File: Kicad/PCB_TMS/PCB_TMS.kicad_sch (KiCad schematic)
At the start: 3 parts

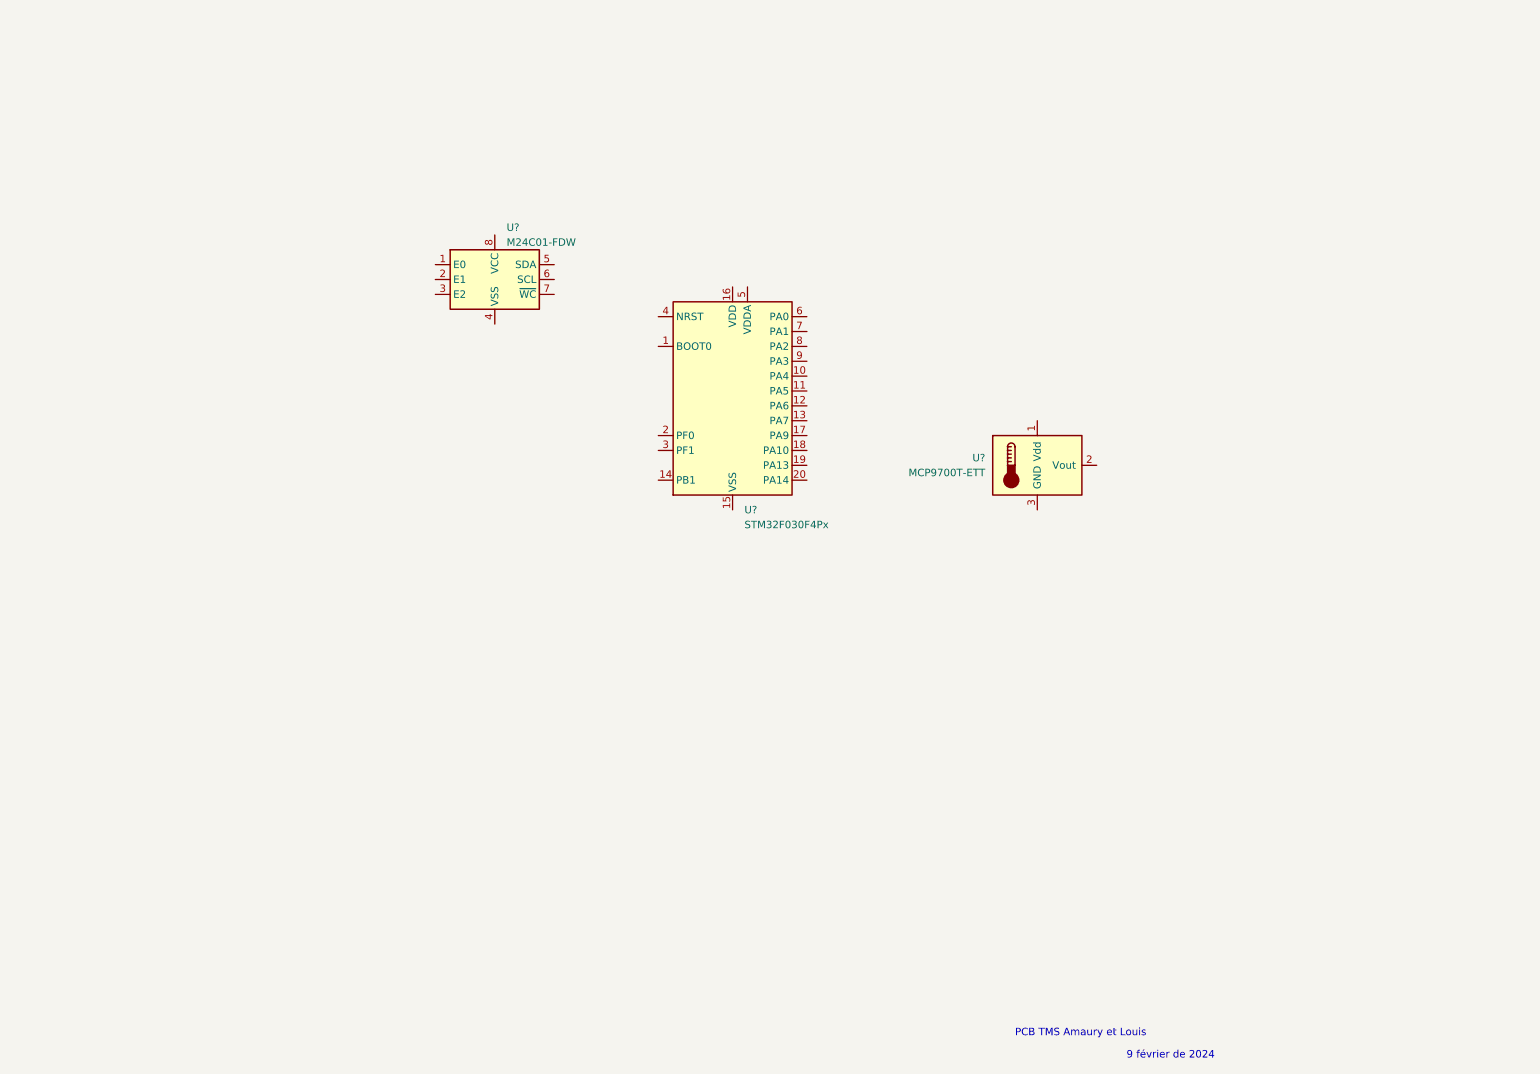
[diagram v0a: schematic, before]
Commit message: Fin schematic
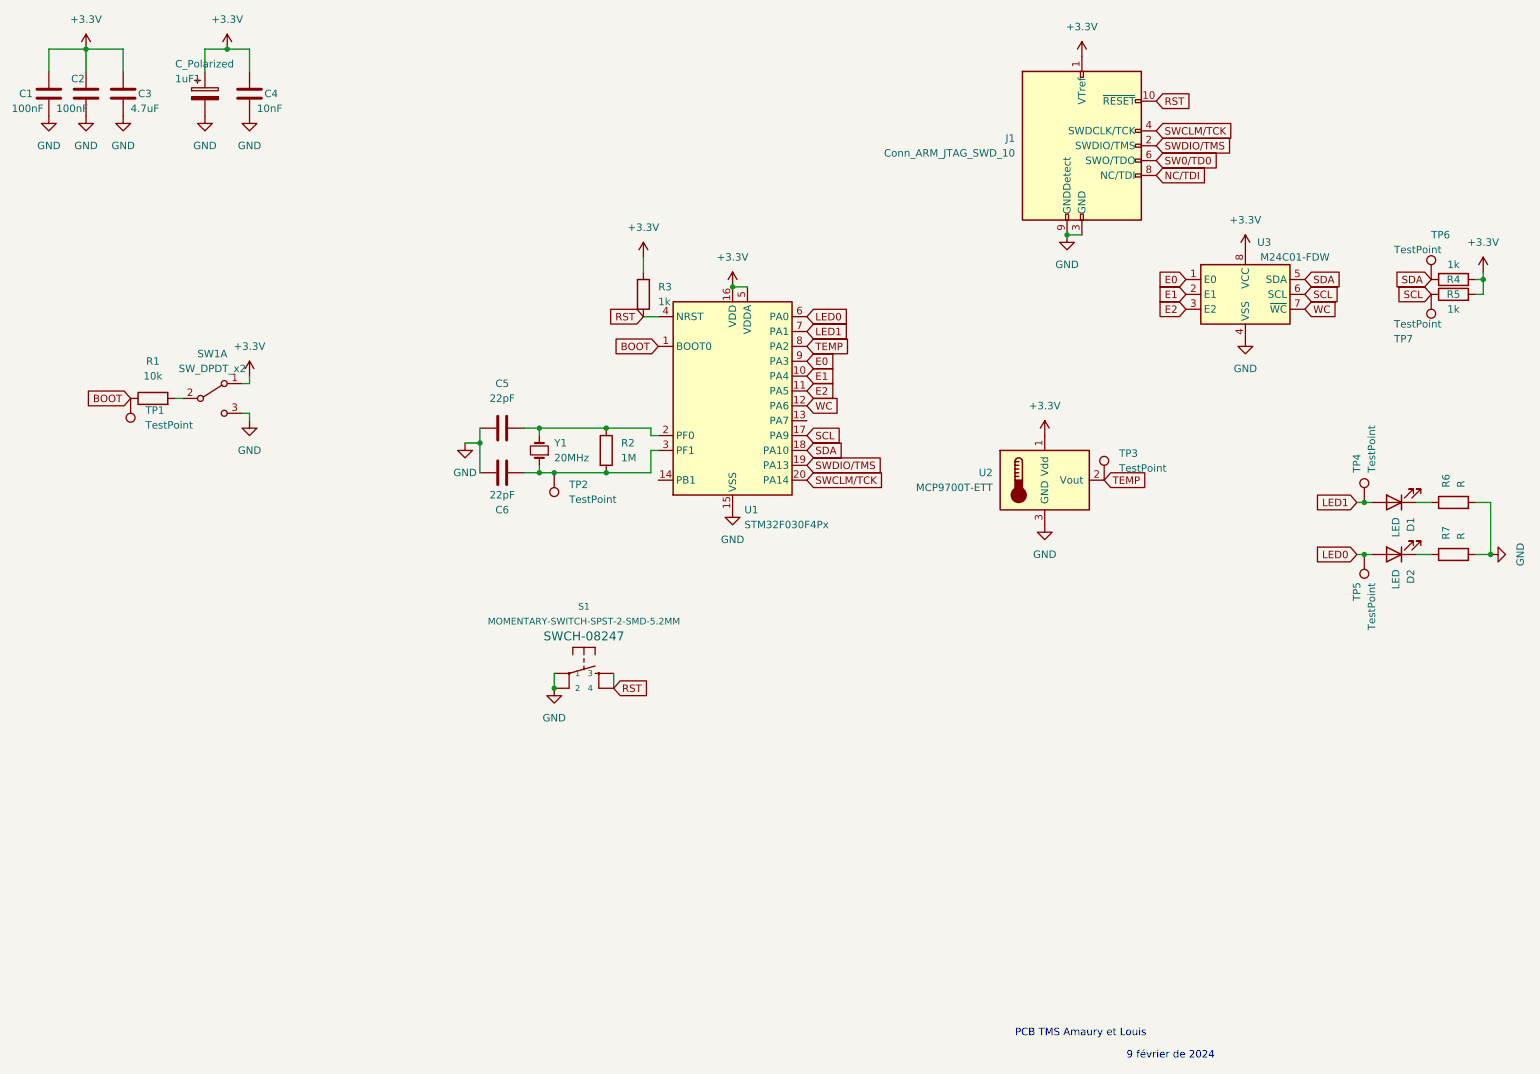
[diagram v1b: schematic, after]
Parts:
- added 1uF1: C_Polarized, symbol Device:C_Polarized
- added C1, C2: 100nF, Capacitor_SMD:C_0201_0603Metric, symbol Device:C
- added C3: 4.7uF, Capacitor_SMD:C_0201_0603Metric, symbol Device:C
- added C4: 10nF, Capacitor_SMD:C_0201_0603Metric, symbol Device:C
- added C5, C6: 22pF, Capacitor_SMD:C_0201_0603Metric, symbol Device:C
- added D1, D2: LED, Diode_SMD:D_0201_0603Metric, symbol Device:LED
- added J1: Conn_ARM_JTAG_SWD_10, Connector_PinHeader_2.54mm:PinHeader_2x05_P2.54mm_Horizontal, symbol Connector:Conn_ARM_JTAG_SWD_10
- added R1: 10k, Resistor_SMD:R_0201_0603Metric, symbol Device:R
- added R2: 1M, Resistor_SMD:R_0201_0603Metric, symbol Device:R
- added R3, R4, R5: 1k, Resistor_SMD:R_0201_0603Metric, symbol Device:R
- added R6, R7: R, Resistor_SMD:R_0201_0603Metric, symbol Device:R
- added S1: MOMENTARY-SWITCH-SPST-2-SMD-5.2MM, Switches:TACTILE_SWITCH_SMD_5.2MM, symbol SparkFun-Switches:MOMENTARY-SWITCH-SPST-2-SMD-5.2MM
- added SW1: SW_DPDT_x2, Switches:TACTILE_SWITCH_SMD_5.2MM, symbol Switch:SW_DPDT_x2
- added TP1, TP2, TP3, TP4, TP5, TP6, TP7: TestPoint, TestPoint:TestPoint_Pad_D2.0mm, symbol Connector:TestPoint
- added Y1: 20MHz, Crystal:Crystal_SMD_HC49-SD_HandSoldering, symbol Device:Crystal_Small
- gave numbers to parts that had none: 3
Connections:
- net E0: now reaches U3.1 (E0)
- net E0: now also U1.9 (PA3)
- net E1: now reaches U3.2 (E1)
- net E1: now also U1.10 (PA4)
- net E2: now reaches U3.3 (E2)
- net E2: now also U1.11 (PA5)
- net GND: now reaches U3.4 (VSS)
- net GND: now also U1.15 (VSS), U2.3 (GND), 1uF1.2, C1.1, C2.1, C3.1, C4.1, C5.1, C6.1, J1.3 (GND), J1.5 (GND), J1.9 (GNDDetect), R6.2, R7.2, S1.1, S1.2, SW1.3 (C)
- net SDA: now reaches U3.5 (SDA)
- net SDA: now also U1.18 (PA10), R4.2, TP6.1
- net SCL: now reaches U3.6 (SCL)
- net SCL: now also U1.17 (PA9), R5.1, TP7.1
- net WC: now reaches U3.7 (~{WC})
- net WC: now also U1.12 (PA6)
- net +3.3V: now reaches U3.8 (VCC)
- net +3.3V: now also U1.16 (VDD), U1.5 (VDDA), U2.1 (Vdd), 1uF1.1, C1.2, C2.2, C3.2, C4.2, J1.1 (VTref), R3.1, R4.1, R5.2, SW1.1 (A)
- net BOOT: now reaches U1.1 (BOOT0)
- net BOOT: now also R1.1, TP1.1
- net SWDIO/TMS: now reaches U1.19 (PA13)
- net SWDIO/TMS: now also J1.2 (SWDIO/TMS)
- net at U1.2 (PF0): now also C5.2, R2.1, Y1.2
- net SWCLM/TCK: now reaches U1.20 (PA14)
- net SWCLM/TCK: now also J1.4 (SWDCLK/TCK)
- net at U1.3 (PF1): now also C6.2, R2.2, TP2.1, Y1.1
- net RST: now reaches U1.4 (NRST)
- net RST: now also J1.10 (~{RESET}), R3.2, S1.3, S1.4
- net LED0: now reaches U1.6 (PA0)
- net LED0: now also D2.2 (A), TP5.1
- net LED1: now reaches U1.7 (PA1)
- net LED1: now also D1.2 (A), TP4.1
- net TEMP: now reaches U1.8 (PA2)
- net TEMP: now also U2.2 (Vout), TP3.1
- new net: D1.1 (K), R6.1
- new net: D2.1 (K), R7.1
- new net: R1.2, SW1.2 (B)
- new net NC/TDI: J1.8 (NC/TDI)
- new net SW0/TD0: J1.6 (SWO/TDO)
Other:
- moved on the sheet: U2, U3

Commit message: Début routage
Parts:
- 1uF1: footprint (none) -> Capacitor_SMD:C_0201_0603Metric
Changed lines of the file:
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@@
       (effects (font (size 1.27 1.27)) (justify left))
     )
-    (property "Footprint" "" (id 2) (at 49.2252 33.02 0)
+    (property "Footprint" "Capacitor_SMD:C_0201_0603Metric" (id 2) (at 49.2252 33.02 0)
       (effects (font (size 1.27 1.27)) hide)
     )
@@
     )
     (path "/2d7759f0-2416-4be2-9d1b-def3393dac33"
-      (reference "1uF1") (unit 1) (value "C_Polarized") (footprint "")
+      (reference "1uF1") (unit 1) (value "C_Polarized") (footprint "Capacitor_SMD:C_0201_0603Metric")
     )
     (path "/6c46b9fc-67e9-4026-b550-82f385903331"

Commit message: Changement d'empreintes
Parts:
- 1uF1, C1, C2, C3, C4, C5, C6: footprint Capacitor_SMD:C_0201_0603Metric -> Capacitor_SMD:C_0603_1608Metric_Pad1.08x0.95mm_HandSolder
- D1, D2: footprint Diode_SMD:D_0201_0603Metric -> Diode_SMD:D_0603_1608Metric_Pad1.05x0.95mm_HandSolder
- J1: footprint Connector_PinHeader_2.54mm:PinHeader_2x05_P2.54mm_Horizontal -> Connector_PinHeader_2.54mm:PinHeader_2x05_P2.54mm_Vertical
- R1, R2, R3, R4, R5, R6, R7: footprint Resistor_SMD:R_0201_0603Metric -> Resistor_SMD:R_0603_1608Metric_Pad0.98x0.95mm_HandSolder
- TP1, TP2, TP3, TP4, TP5, TP6, TP7: footprint TestPoint:TestPoint_Pad_D2.0mm -> TestPoint:TestPoint_Pad_D1.0mm

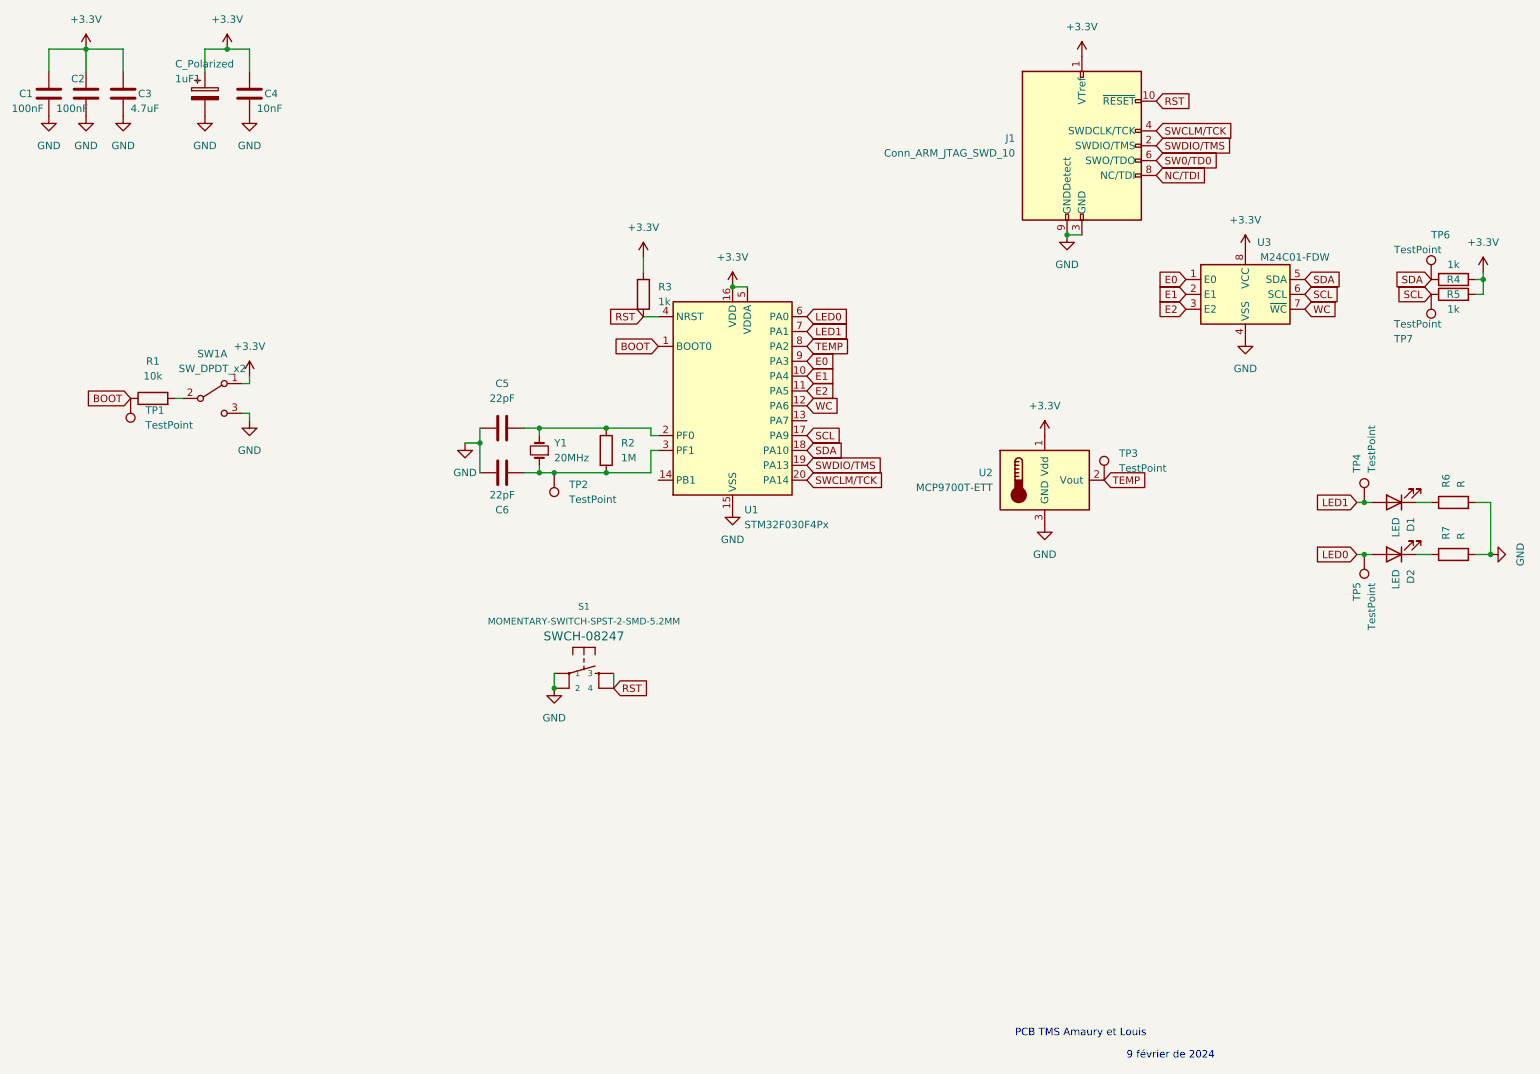
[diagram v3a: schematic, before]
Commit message: PCB Routage fini
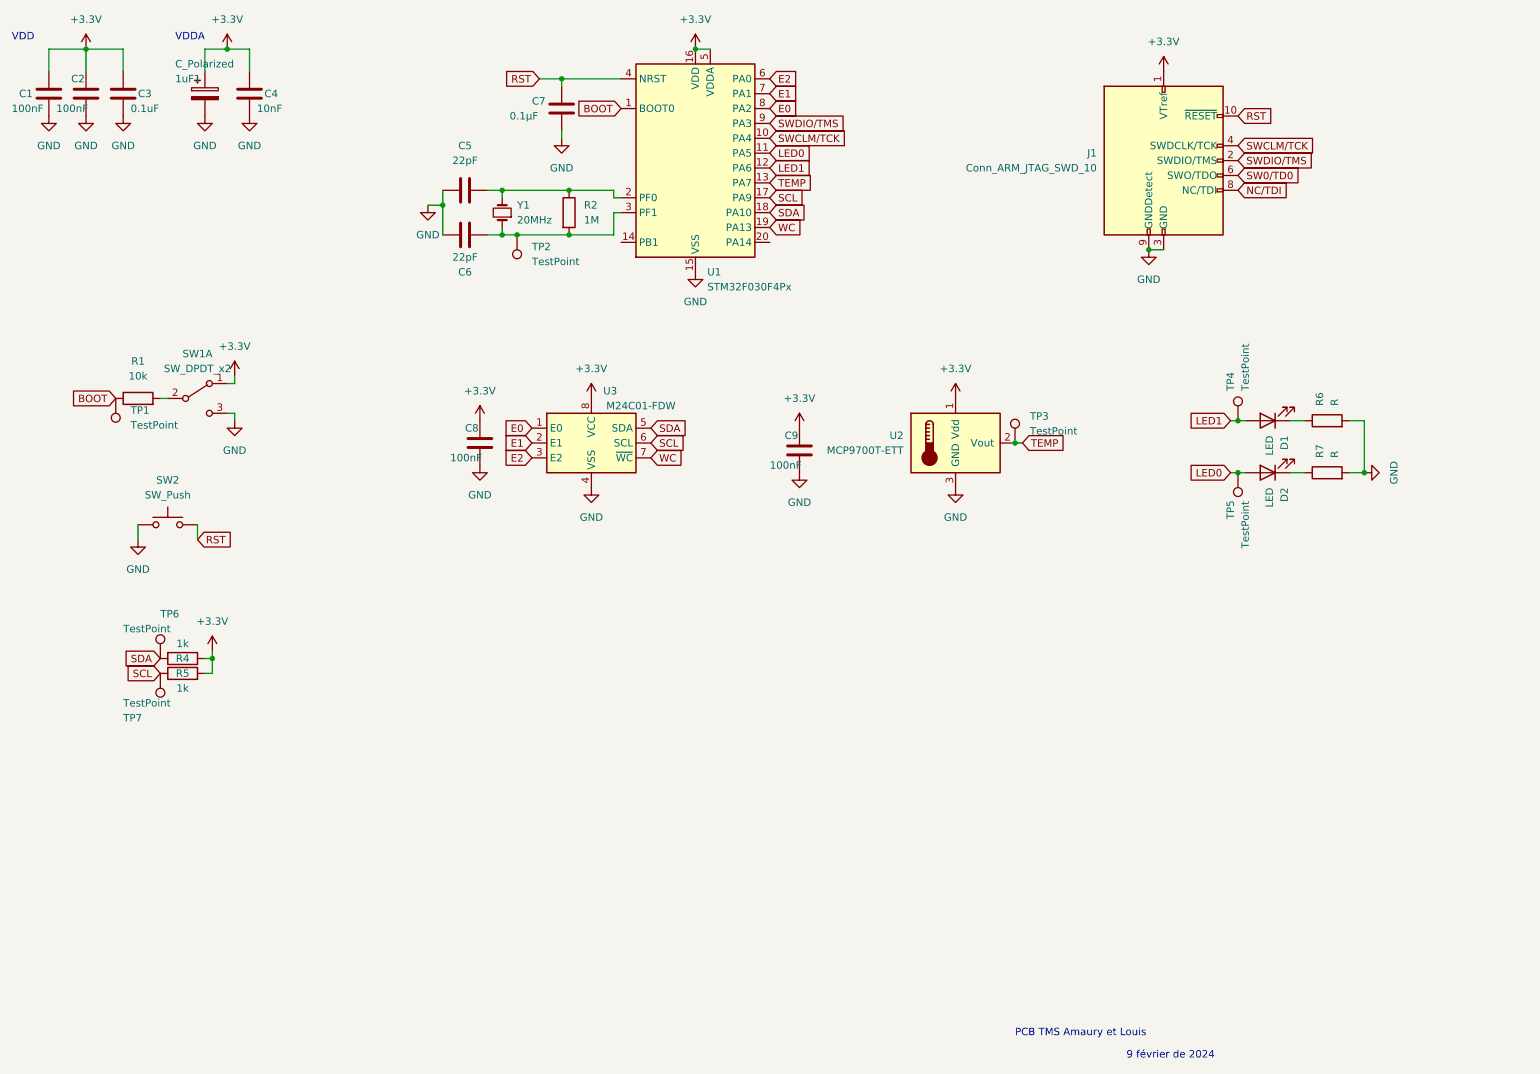
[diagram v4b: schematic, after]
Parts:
- removed R3: 1k, Resistor_SMD:R_0603_1608Metric_Pad0.98x0.95mm_HandSolder, symbol Device:R
- removed S1: MOMENTARY-SWITCH-SPST-2-SMD-5.2MM, Switches:TACTILE_SWITCH_SMD_5.2MM, symbol SparkFun-Switches:MOMENTARY-SWITCH-SPST-2-SMD-5.2MM
- added C7: 0.1µF, Capacitor_SMD:C_0603_1608Metric_Pad1.08x0.95mm_HandSolder, symbol Device:C
- added C8, C9: 100nF, Capacitor_SMD:C_0603_1608Metric_Pad1.08x0.95mm_HandSolder, symbol Device:C
- added SW2: SW_Push, Button_Switch_SMD:SW_SPST_SKQG_WithStem, symbol Switch:SW_Push
- C3: value 4.7uF -> 0.1uF
- SW1: footprint Switches:TACTILE_SWITCH_SMD_5.2MM -> Connector_PinHeader_2.54mm:PinHeader_1x03_P2.54mm_Vertical
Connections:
- net +3.3V: now also C8.2, C9.2
- net E0: now also U1.8 (PA2); no longer U1.9 (PA3)
- net E1: now also U1.7 (PA1); no longer U1.10 (PA4)
- net E2: now also U1.6 (PA0); no longer U1.11 (PA5)
- net GND: now also C7.1, C8.1, C9.1, SW2.1
- net LED0: now also U1.11 (PA5); no longer U1.6 (PA0)
- net LED1: now also U1.12 (PA6); no longer U1.7 (PA1)
- net RST: now also C7.2, SW2.2
- net SWCLM/TCK: now also U1.10 (PA4); no longer U1.20 (PA14)
- net SWDIO/TMS: now also U1.9 (PA3); no longer U1.19 (PA13)
- net TEMP: now also U1.13 (PA7); no longer U1.8 (PA2)
- net WC: now also U1.19 (PA13); no longer U1.12 (PA6)
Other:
- note added: "VDD"
- note added: "VDDA"
- moved on the sheet: C5, C6, D1, D2, J1, R1, R2, R4, R5, R6, R7, SW1A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

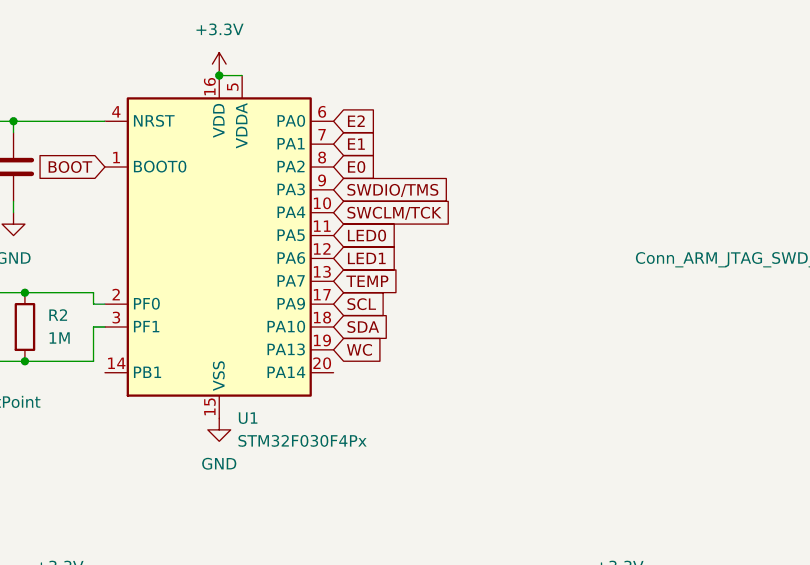
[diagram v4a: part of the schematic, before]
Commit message: correction PCB
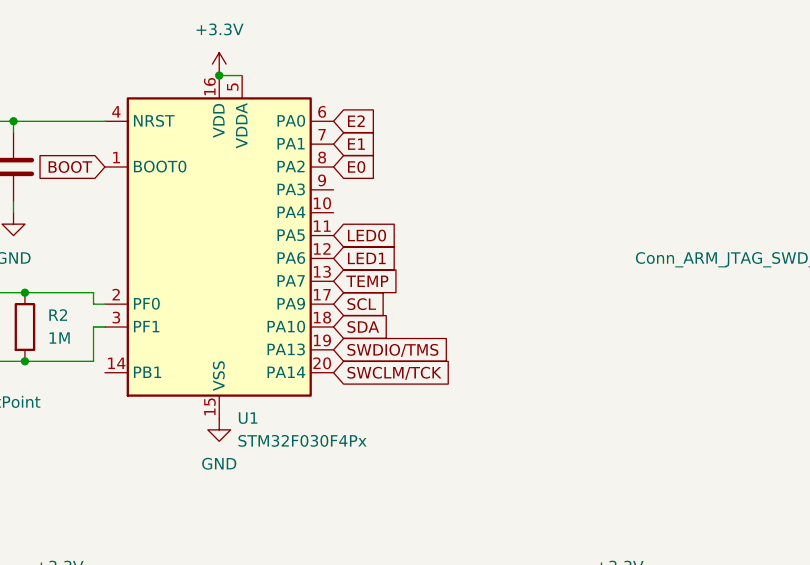
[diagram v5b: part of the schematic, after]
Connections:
- net SWCLM/TCK: now also U1.20 (PA14); no longer U1.10 (PA4)
- net SWDIO/TMS: now also U1.19 (PA13); no longer U1.9 (PA3)
- net WC: no longer U1.19 (PA13)
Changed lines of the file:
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@@
     )
   )
-  (global_label "SWCLM{slash}TCK" (shape input) (at 144.78 36.83 0) (fields_autoplaced)
+  (global_label "SWCLM{slash}TCK" (shape input) (at 144.78 54.61 0) (fields_autoplaced)
     (effects (font (size 1.27 1.27)) (justify left))
-    (property "Références Inter-Feuilles" "${INTERSHEET_REFS}" (id 0) (at 158.4417 36.7506 0)
+    (property "Références Inter-Feuilles" "${INTERSHEET_REFS}" (id 0) (at 158.4417 54.5306 0)
       (effects (font (size 1.27 1.27)) (justify left) hide)
     )
   )
-  (global_label "SWDIO{slash}TMS" (shape input) (at 144.78 34.29 0) (fields_autoplaced)
+  (global_label "SWDIO{slash}TMS" (shape input) (at 144.78 52.07 0) (fields_autoplaced)
     (effects (font (size 1.27 1.27)) (justify left))
-    (property "Références Inter-Feuilles" "${INTERSHEET_REFS}" (id 0) (at 158.0183 34.2106 0)
+    (property "Références Inter-Feuilles" "${INTERSHEET_REFS}" (id 0) (at 158.0183 51.9906 0)
       (effects (font (size 1.27 1.27)) (justify left) hide)
     )
@@
       (effects (font (size 1.27 1.27)) (justify left) hide)
     )
-  )
-  (global_label "WC" (shape input) (at 144.78 52.07 0) (fields_autoplaced)
-    (effects (font (size 1.27 1.27)) (justify left))
-    (property "Références Inter-Feuilles" "${INTERSHEET_REFS}" (id 0) (at 149.9145 51.9906 0)
-      (effects (font (size 1.27 1.27)) (justify left) hide)
-    )
